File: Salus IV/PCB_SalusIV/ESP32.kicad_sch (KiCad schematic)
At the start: 21 parts, among them J4 Pruebas

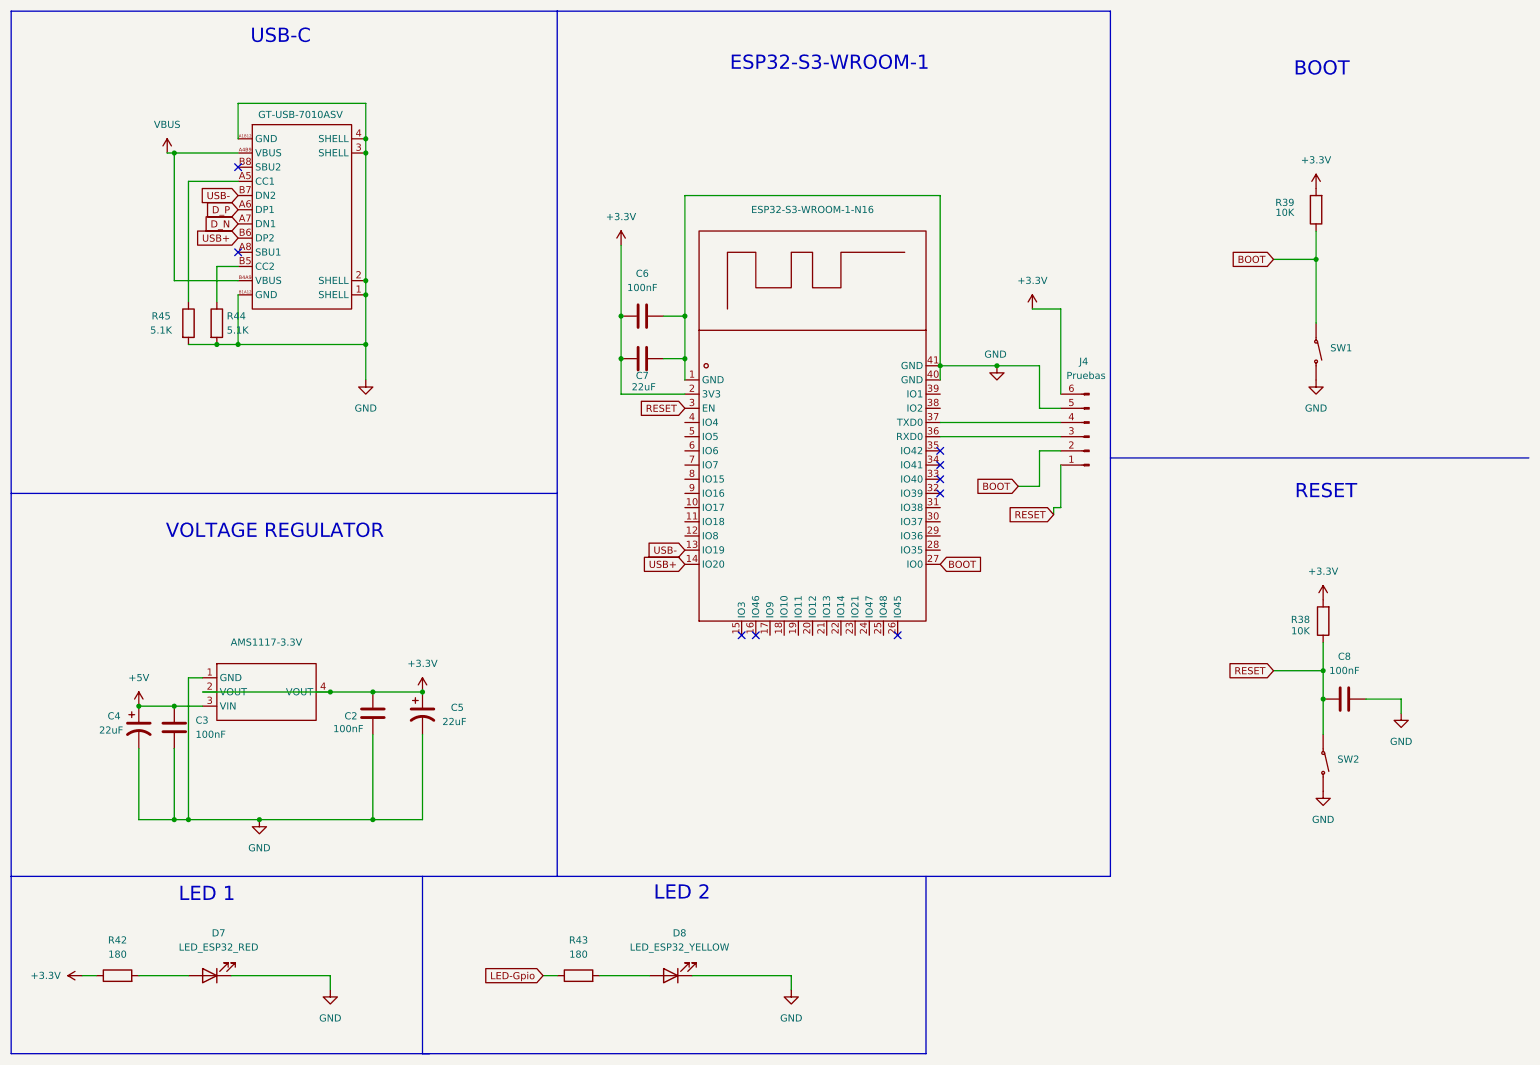
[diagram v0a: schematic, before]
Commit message: Se agregan cambios antes de agregar arrays
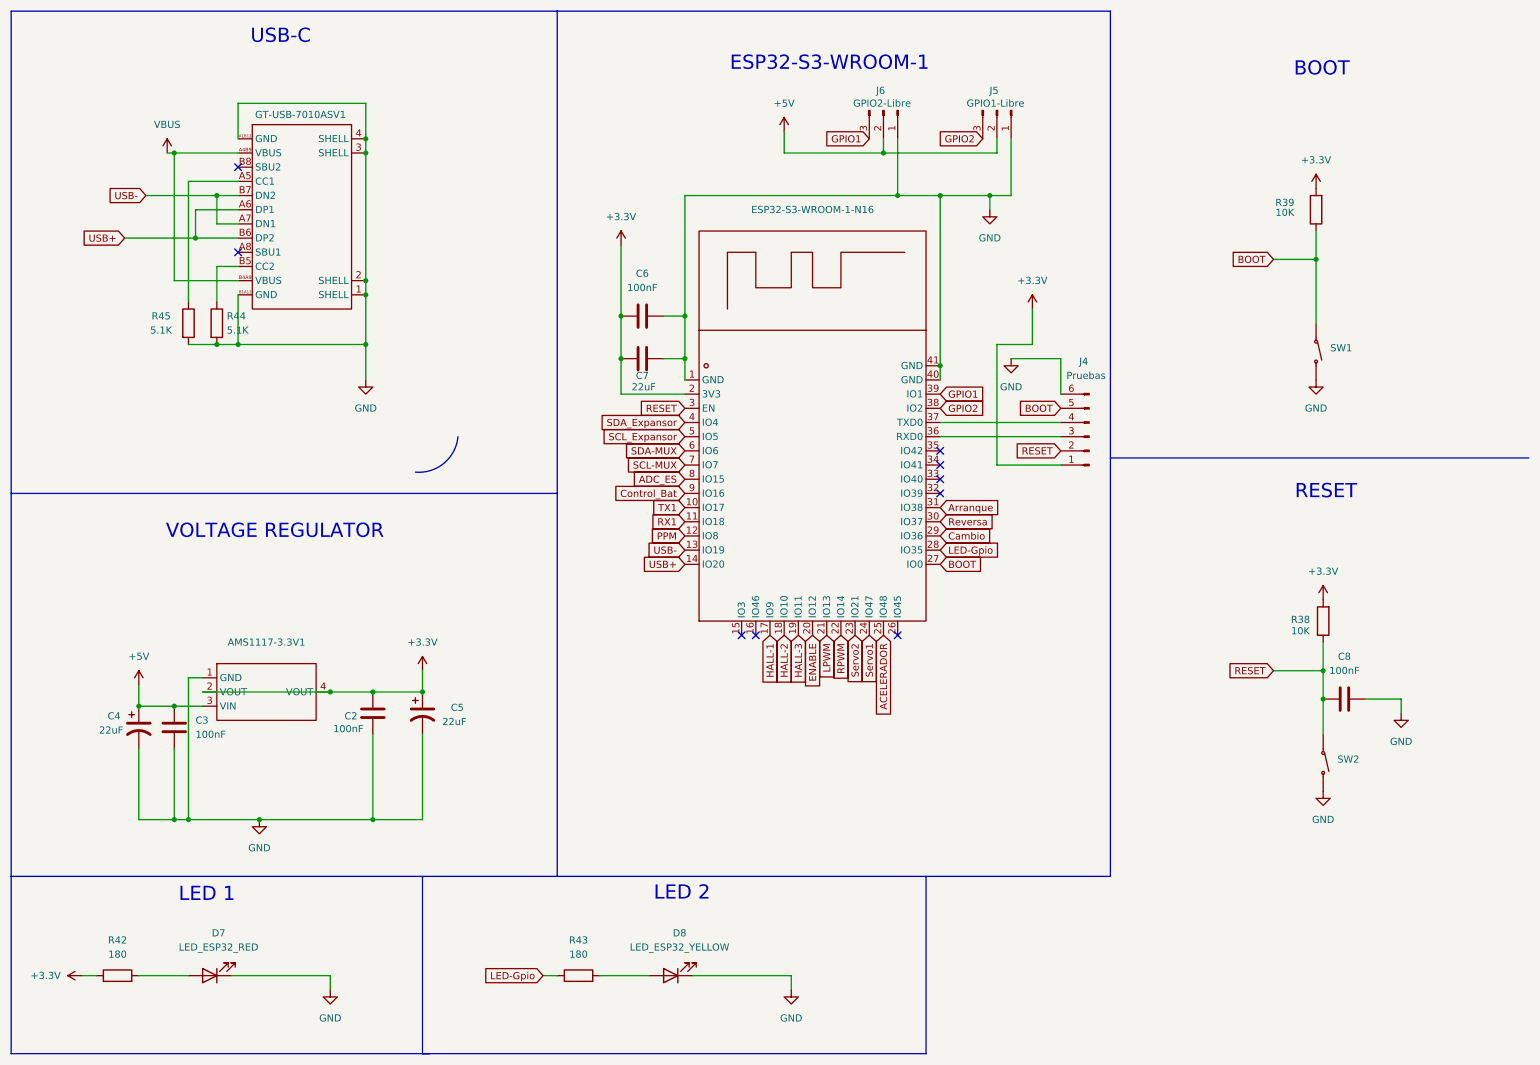
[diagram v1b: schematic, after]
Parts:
- added J5: GPIO1-Libre, Connector_PinHeader_2.54mm:PinHeader_1x03_P2.54mm_Vertical, symbol Connector:Conn_01x03_Pin
- added J6: GPIO2-Libre, Connector_PinHeader_2.54mm:PinHeader_1x03_P2.54mm_Vertical, symbol Connector:Conn_01x03_Pin
- renumbered AMS1117-3.3V to AMS1117-3.3V1, GT-USB-7010ASV to GT-USB-7010ASV1
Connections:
- net D_N is gone; now on net USB-: GT-USB-7010ASV1.A7 (DN1)
- net D_P is gone; now on net USB+: GT-USB-7010ASV1.A6 (DP1)
- net +3.3V: now also J4.1 (Pin_1); no longer J4.6 (Pin_6)
- net +5V: now also J5.2 (Pin_2), J6.2 (Pin_2)
- net BOOT: now also J4.5 (Pin_5); no longer J4.2 (Pin_2)
- net GND: now also J4.6 (Pin_6), J5.1 (Pin_1), J6.1 (Pin_1); no longer J4.5 (Pin_5)
- net LED-Gpio: now also ESP32-S3-WROOM-1-N16.28 (IO35)
- net RESET: now also J4.2 (Pin_2); no longer J4.1 (Pin_1)
- net TX1: now reaches ESP32-S3-WROOM-1-N16.10 (IO17)
- net RX1: now reaches ESP32-S3-WROOM-1-N16.11 (IO18)
- net PPM: now reaches ESP32-S3-WROOM-1-N16.12 (IO8)
- net HALL-1: now reaches ESP32-S3-WROOM-1-N16.17 (IO9)
- net HALL-2: now reaches ESP32-S3-WROOM-1-N16.18 (IO10)
- net HALL-3: now reaches ESP32-S3-WROOM-1-N16.19 (IO11)
- net ENABLE: now reaches ESP32-S3-WROOM-1-N16.20 (IO12)
- net LPWM: now reaches ESP32-S3-WROOM-1-N16.21 (IO13)
- net RPWM: now reaches ESP32-S3-WROOM-1-N16.22 (IO14)
- net Servo2: now reaches ESP32-S3-WROOM-1-N16.23 (IO21)
- net Servo1: now reaches ESP32-S3-WROOM-1-N16.24 (IO47)
- net ACELERADOR: now reaches ESP32-S3-WROOM-1-N16.25 (IO48)
- net Cambio: now reaches ESP32-S3-WROOM-1-N16.29 (IO36)
- net Reversa: now reaches ESP32-S3-WROOM-1-N16.30 (IO37)
- net Arranque: now reaches ESP32-S3-WROOM-1-N16.31 (IO38)
- net GPIO2: now reaches ESP32-S3-WROOM-1-N16.38 (IO2)
- net GPIO2: now also J5.3 (Pin_3)
- net GPIO1: now reaches ESP32-S3-WROOM-1-N16.39 (IO1)
- net GPIO1: now also J6.3 (Pin_3)
- net SDA_Expansor: now reaches ESP32-S3-WROOM-1-N16.4 (IO4)
- net SCL_Expansor: now reaches ESP32-S3-WROOM-1-N16.5 (IO5)
- net SDA-MUX: now reaches ESP32-S3-WROOM-1-N16.6 (IO6)
- net SCL-MUX: now reaches ESP32-S3-WROOM-1-N16.7 (IO7)
- net ADC_ES: now reaches ESP32-S3-WROOM-1-N16.8 (IO15)
- net Control_Bat: now reaches ESP32-S3-WROOM-1-N16.9 (IO16)
